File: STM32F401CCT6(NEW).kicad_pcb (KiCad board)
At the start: 2 copper layers, 37 parts, among them J1 USB_OTG, J2 Conn_02x03_Odd_Even, J3 Conn_01x20_des, J4 Conn_01x05_desc, J5 Conn_01x20, SW1 SW_Push, U1 MIC5219-3.3, U2 STM32F401CCT6, U3 USBLC6-2SC6, Y1 32.786K, Y2 8MHz

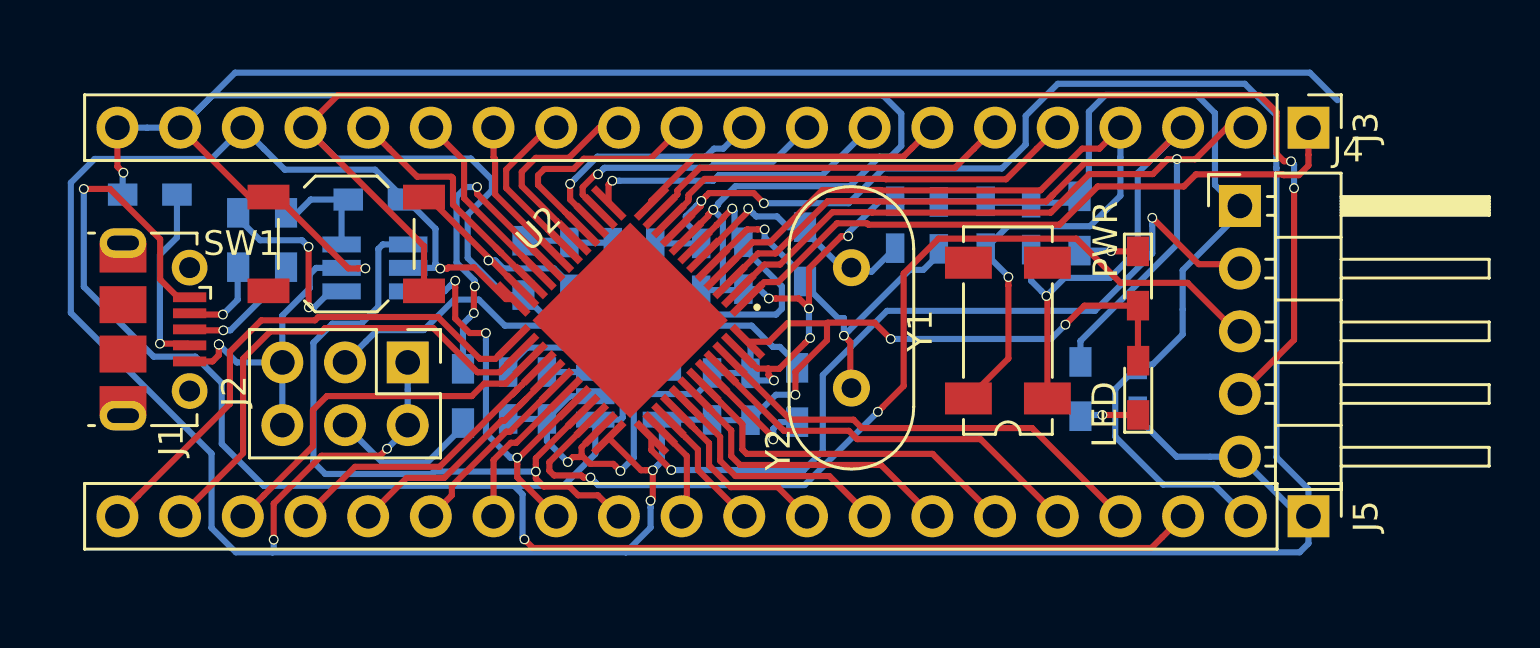
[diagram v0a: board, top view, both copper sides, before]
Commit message: Finish routing
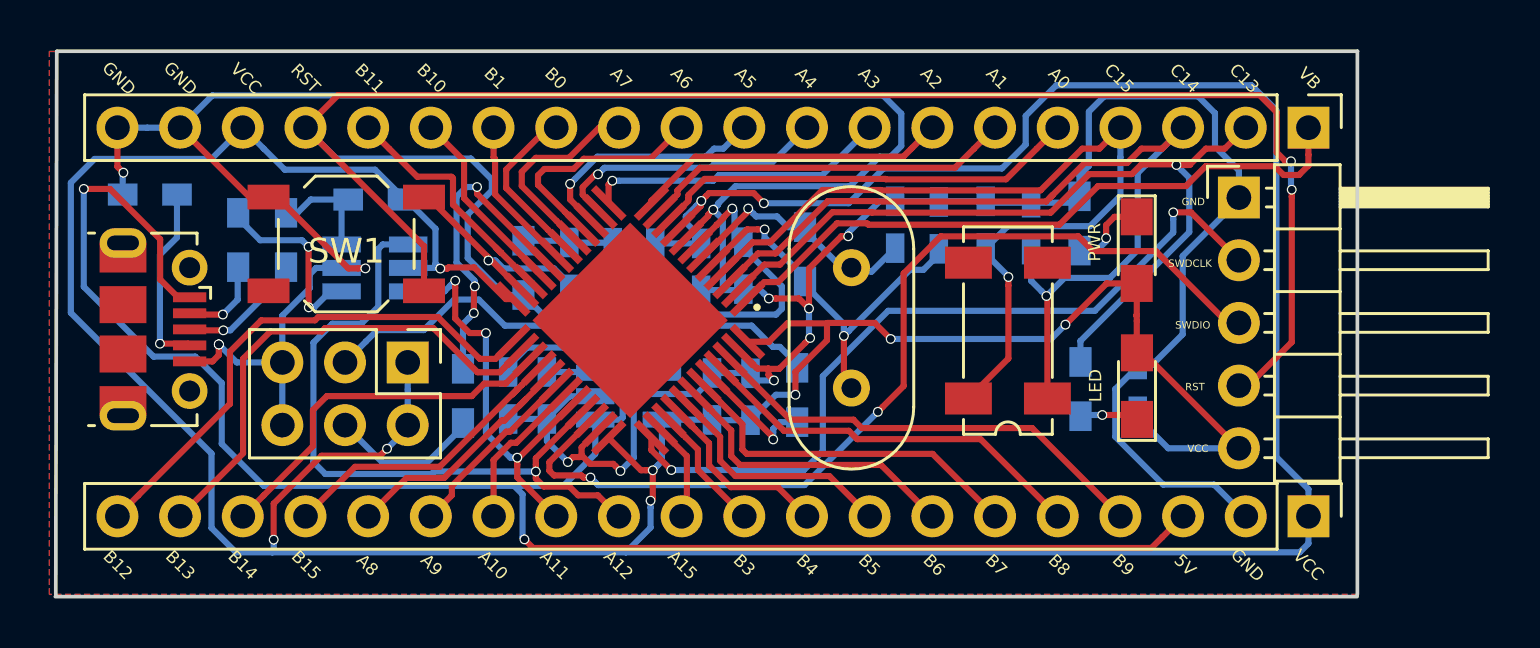
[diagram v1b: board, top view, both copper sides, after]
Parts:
- removed the LED at (117.4, 114.2)
- removed the PWR at (117.4, 109.7)
- added LED: LED_ALT, LEDs:LED_0805_HandSoldering, F.Cu at (117.4, 114.1)
- added PWR: LED_ALT, LEDs:LED_0805_HandSoldering, F.Cu at (117.4, 108.6)
- moved J4 0.34 mm to (121.5, 106.5)
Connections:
- J1 pad 6: Net-(J1-Pad6) -> (no net)
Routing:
- net GND: track 214.9 -> 165.5 mm
- net VCC: track 199.3 -> 201.6 mm
- net Net-(D1-Pad1): track 2.42 -> 3.27 mm
- net /PC13: track 33.1 -> 33.9 mm
- added copper zone on B.Cu, net GND
- added copper zone on F.Cu, net GND
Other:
- board outline added: 52.8 x 22.1 mm
- board text added: "5V"
- board text added: "A0"
- board text added: "A1"
- board text added: "A10"
- board text added: "A11"
- board text added: "A12"
- board text added: "A15"
- board text added: "A2"
- board text added: "A3"
- board text added: "A4"
- board text added: "A5"
- board text added: "A6"
- board text added: "A7"
- board text added: "A8"
- board text added: "A9"
- board text added: "B0"
- board text added: "B1"
- board text added: "B10"
- board text added: "B11"
- board text added: "B12"
- board text added: "B13"
- board text added: "B14"
- board text added: "B15"
- board text added: "B3"
- board text added: "B4"
- board text added: "B5"
- board text added: "B6"
- board text added: "B7"
- board text added: "B8"
- board text added: "B9"
- board text added: "C13"
- board text added: "C14"
- board text added: "C15"
- board text added: "GND"
- board text added: "RST"
- board text added: "SWDCLK"
- board text added: "SWDIO"
- board text added: "VB"
- board text added: "VCC"
